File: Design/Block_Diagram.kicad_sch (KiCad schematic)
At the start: 0 parts

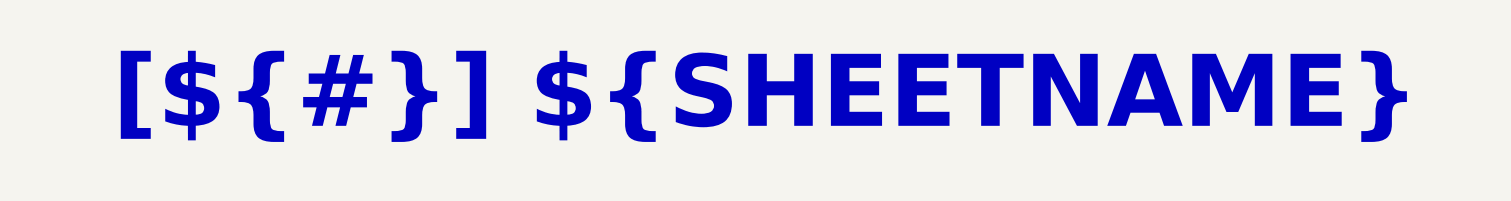
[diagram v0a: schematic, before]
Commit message: new frame work for the design
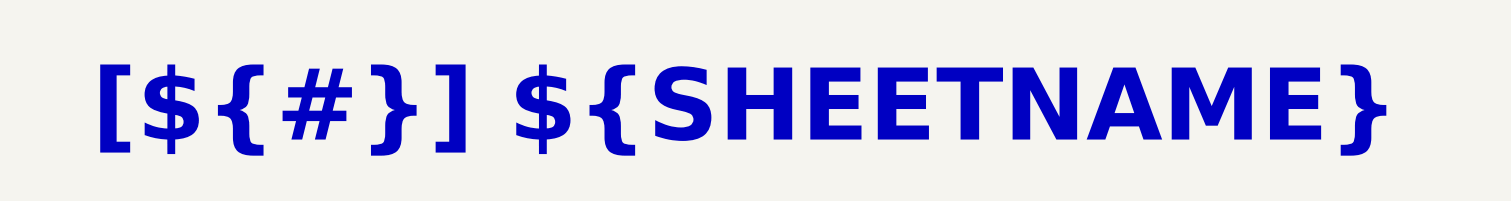
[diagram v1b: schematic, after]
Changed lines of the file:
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@@
 	(text "[${#}] ${SHEETNAME}"
 		(exclude_from_sim no)
-		(at 140.716 22.86 0)
+		(at 138.43 24.384 0)
 		(effects
 			(font
